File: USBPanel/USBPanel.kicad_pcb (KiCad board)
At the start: 6 copper layers, 36 x 38 mm, 68 parts, among them J1 PORT1, J2 PORT2, J3 PWR, J4 USB_UFP, J5 SINK, J6 I2Ct, J7 I2Cc, Q1 ISZ0702NLS, Q2 ISZ0702NLS, Q3 NX138BK, Q4 NX138BK, Q5 NX138BK, U1 TPS25751S, U2 VBUS54CV-HSF, U3 M24512E-FMN, U4 TPS25810, U5 TS3USB31, U6 74LVC1T45DW

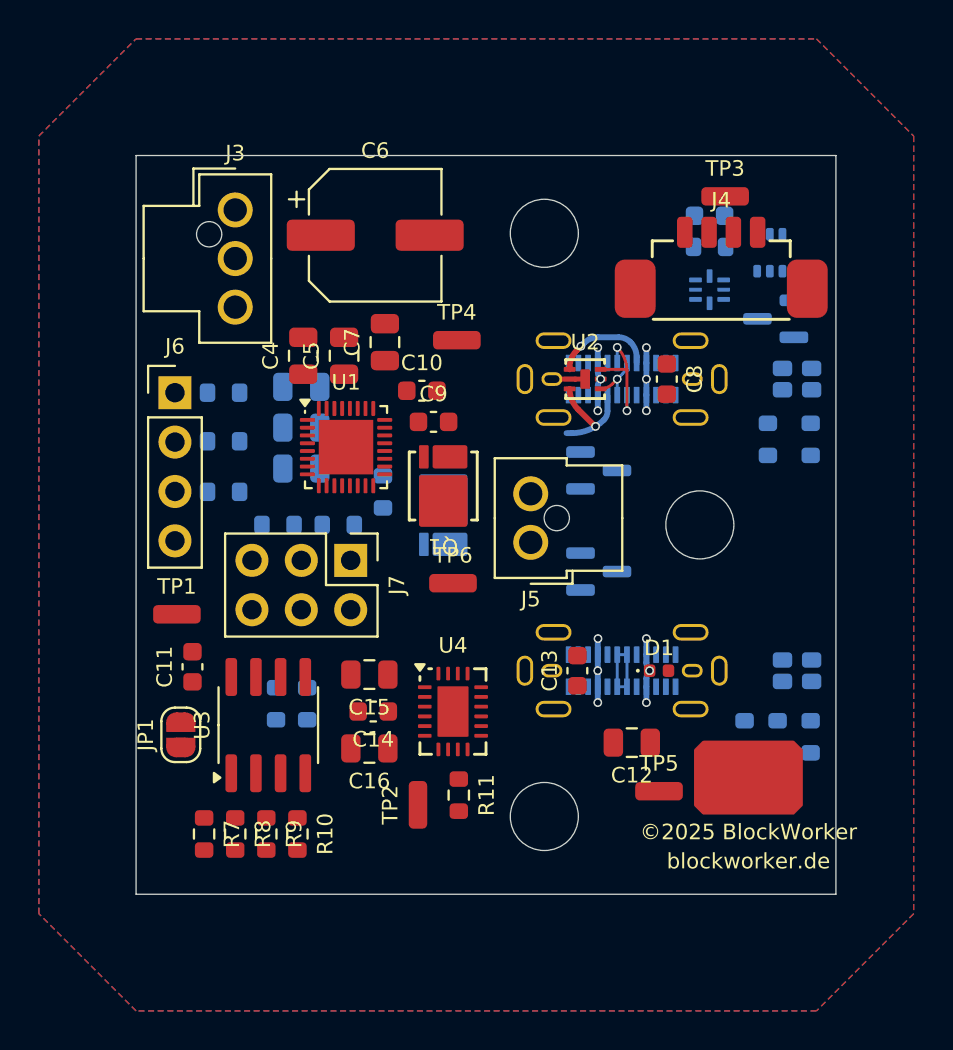
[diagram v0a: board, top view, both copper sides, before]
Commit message: USBPanel PCB complete
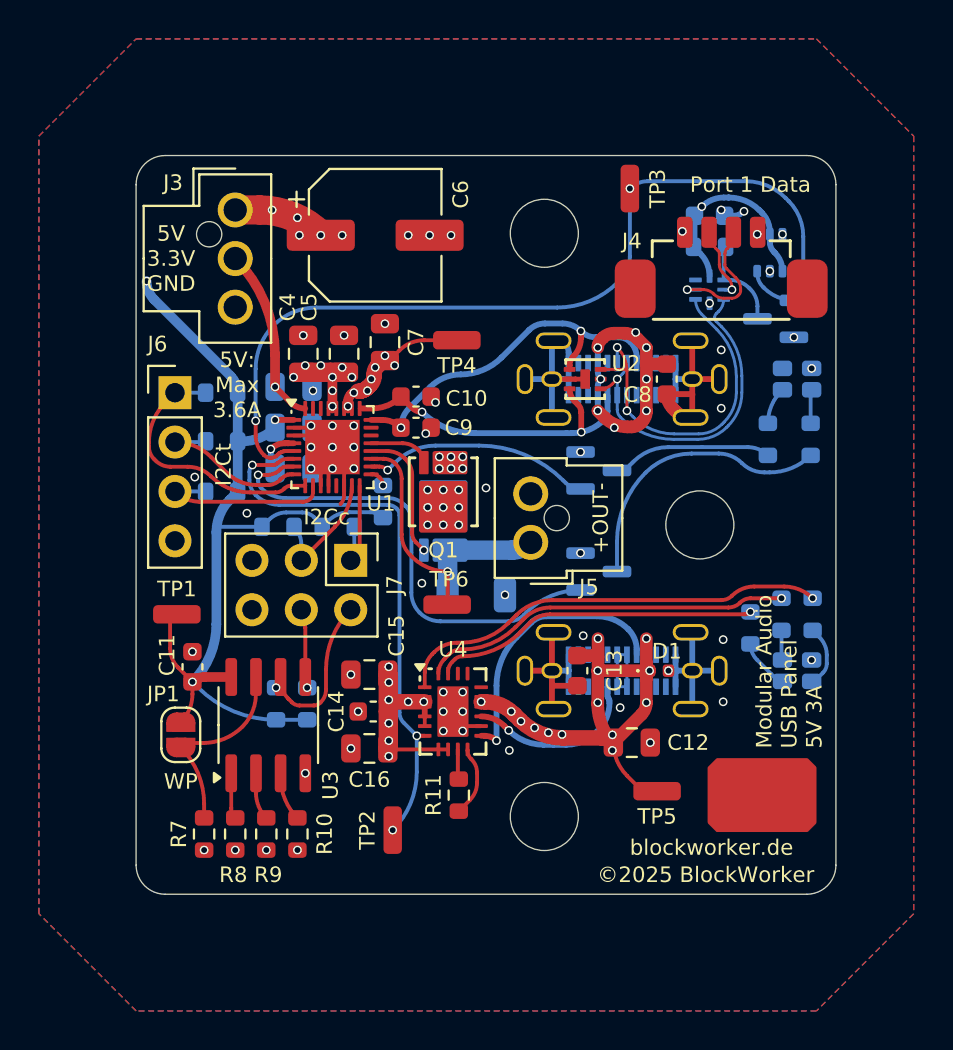
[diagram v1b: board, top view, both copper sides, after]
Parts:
- added C18: 10μF 50V, Capacitor_SMD:C_1206_3216Metric, B.Cu at (147.5, 103.6)
- moved R17 6.58 mm to (163.2, 104.6), turned to -90 degrees
- moved R15 6.30 mm to (164.8, 104.6), turned to -90 degrees
- moved R16 5.77 mm to (161.6, 105.3), turned to -90 degrees
- moved TP3 4.92 mm to (155.4, 82.7), turned to -90 degrees
- moved TP2 1.84 mm to (143.2, 115.7)
- moved REF** 1.14 mm to (162.2, 113.9)
- moved TP6 1.14 mm to (146.0, 104.1)
- moved C9 0.95 mm to (144.4, 95.0)
- moved U1 0.70 mm to (140.1, 96.0)
- moved R3 0.50 mm to (142.7, 98.8)
- moved C10 0.42 mm to (144.4, 93.4)
- moved C1 0.40 mm to (138.1, 92.9)
- moved C2 0.40 mm to (138.1, 95.0)
- moved C3 0.40 mm to (138.1, 97.1)
- moved Q1 0.30 mm to (145.8, 98.3)
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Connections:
- net Net-(D1-A1) renamed /PORT2_VBUS
- net Net-(Q1-S) renamed /PORT1_VBUS
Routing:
- net +3.3V: track 0.00 -> 95.6 mm, vias 0 -> 4
- net GND: track 1.21 -> 54.1 mm, vias 0 -> 55
- net /PORT1_UFP: track 0.00 -> 48.8 mm, vias 0 -> 2
- net /PORT2_EN: track 0.00 -> 28.9 mm, vias 0 -> 3
- net /PORT2_VBUS: track 6.67 -> 33.7 mm, vias 6 -> 14
- net Net-(Q4-G): track 0.00 -> 24.8 mm, vias 0 -> 1
- net Net-(U4-~{FAULT}): track 0.00 -> 22.5 mm, vias 0 -> 1
- net +5V: track 0.00 -> 19.4 mm, vias 0 -> 24
- net Net-(U4-~{LD_DET}): track 0.00 -> 19.1 mm, vias 0 -> 1
- net /PORT1_VBUS: track 6.58 -> 25.1 mm, vias 6 -> 21
- net Net-(U4-~{UFP}): track 0.00 -> 16.7 mm, vias 0 -> 1
- net Net-(J5-Pin_1): track 0.00 -> 16.6 mm, vias 0 -> 1
- net Net-(Q4-D): track 0.00 -> 14.7 mm
- net /PORT1_D+: track 2.84 -> 17.2 mm
- net Net-(J2-CC1): track 0.00 -> 14.2 mm, vias 0 -> 1
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- added copper zone on In2.Cu, net /PORT1_VBUS
- added copper zone on In3.Cu, net /PORT1_VBUS
- added copper zone on In2.Cu, net /PORT2_VBUS
- added copper zone on In3.Cu, net /PORT2_VBUS
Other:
- outline, holes or cut-outs redrawn
- board text added: "+OUT-"
- board text added: "5V 3.3V GND"
- board text added: "5V: Max 3.6A"
- board text added: "I2Cc"
- board text added: "I2Ct"
- board text added: "Modular Audio USB Panel 5V 3A"
- board text added: "Port 1 5V 3A USB 2.0"
- board text added: "Port 1 Data"
- board text added: "Port 2 5V 3A No Data Off if P1 active"
- board text added: "WP"
